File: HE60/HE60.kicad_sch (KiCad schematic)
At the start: 335 parts, among them J1 TYPE-C-31-M-12, J2 SWD, J3 Conn_01x09_MountingPin, J4 Conn_01x06_MountingPin, SW1 TS-1187A-B-A-B, SW2 TS-1187A-B-A-B, U1 USBLC6-2SC6, U2 TLV75733PDBV, U3 XC6206P332MR-G, U4 AT32F405RCT7, Y1 X322512MSB4SI

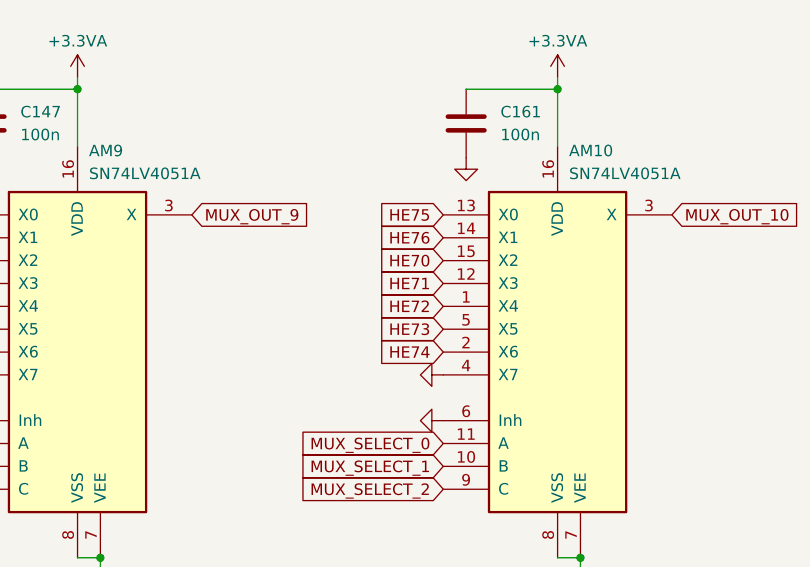
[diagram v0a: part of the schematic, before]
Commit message: add models for 1u
https://grabcad.com/library/cherry-mx-switches-mx-1
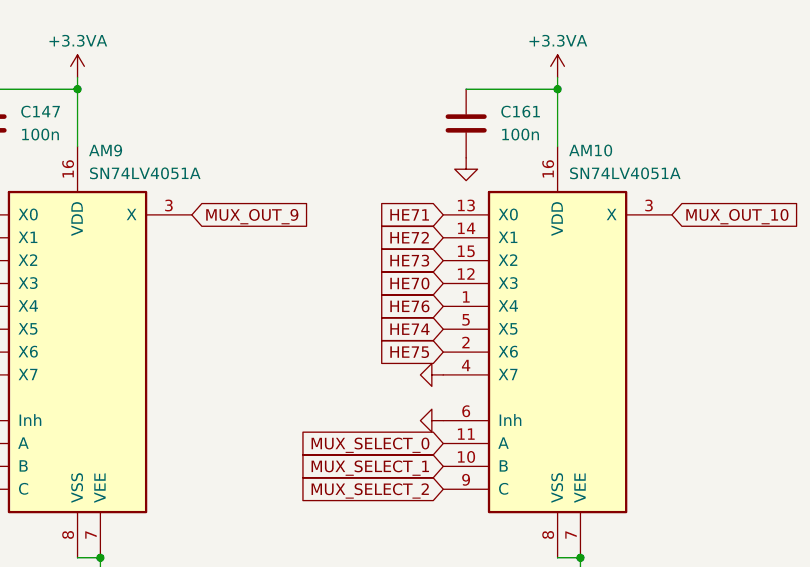
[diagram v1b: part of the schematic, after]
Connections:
- net HE70: now also AM10.12 (X3); no longer AM10.15 (X2)
- net HE71: now also AM10.13 (X0); no longer AM10.12 (X3)
- net HE72: now also AM10.14 (X1); no longer AM10.1 (X4)
- net HE73: now also AM10.15 (X2); no longer AM10.5 (X5)
- net HE74: now also AM10.5 (X5); no longer AM10.2 (X6)
- net HE75: now also AM10.2 (X6); no longer AM10.13 (X0)
- net HE76: now also AM10.1 (X4); no longer AM10.14 (X1)
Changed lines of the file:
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@@
 	(global_label "HE75"
 		(shape input)
-		(at 476.25 208.28 180)
+		(at 476.25 223.52 180)
 		(fields_autoplaced yes)
 		(effects
@@
 		)
 		(property "Intersheetrefs" "${INTERSHEET_REFS}"
-			(at 468.3663 208.28 0)
+			(at 468.3663 223.52 0)
 			(effects
 				(font
@@
 	(global_label "HE74"
 		(shape input)
-		(at 476.25 223.52 180)
+		(at 476.25 220.98 180)
 		(fields_autoplaced yes)
 		(effects
@@
 		)
 		(property "Intersheetrefs" "${INTERSHEET_REFS}"
-			(at 468.3663 223.52 0)
+			(at 468.3663 220.98 0)
 			(effects
 				(font
@@
 	(global_label "HE73"
 		(shape input)
-		(at 476.25 220.98 180)
+		(at 476.25 213.36 180)
 		(fields_autoplaced yes)
 		(effects
@@
 		)
 		(property "Intersheetrefs" "${INTERSHEET_REFS}"
-			(at 468.3663 220.98 0)
+			(at 468.3663 213.36 0)
 			(effects
 				(font
@@
 	(global_label "HE72"
 		(shape input)
-		(at 476.25 218.44 180)
+		(at 476.25 210.82 180)
 		(fields_autoplaced yes)
 		(effects
@@
 		)
 		(property "Intersheetrefs" "${INTERSHEET_REFS}"
-			(at 468.3663 218.44 0)
+			(at 468.3663 210.82 0)
 			(effects
 				(font
@@
 	(global_label "HE76"
 		(shape input)
-		(at 476.25 210.82 180)
+		(at 476.25 218.44 180)
 		(fields_autoplaced yes)
 		(effects
@@
 		)
 		(property "Intersheetrefs" "${INTERSHEET_REFS}"
-			(at 468.3663 210.82 0)
+			(at 468.3663 218.44 0)
 			(effects
 				(font
@@
 	(global_label "HE70"
 		(shape input)
-		(at 476.25 213.36 180)
+		(at 476.25 215.9 180)
 		(fields_autoplaced yes)
 		(effects
@@
 		)
 		(property "Intersheetrefs" "${INTERSHEET_REFS}"
-			(at 468.3663 213.36 0)
+			(at 468.3663 215.9 0)
 			(effects
 				(font
@@
 	(global_label "HE71"
 		(shape input)
-		(at 476.25 215.9 180)
+		(at 476.25 208.28 180)
 		(fields_autoplaced yes)
 		(effects
@@
 		)
 		(property "Intersheetrefs" "${INTERSHEET_REFS}"
-			(at 468.3663 215.9 0)
+			(at 468.3663 208.28 0)
 			(effects
 				(font
